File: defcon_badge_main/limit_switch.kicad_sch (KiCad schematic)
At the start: 5 parts

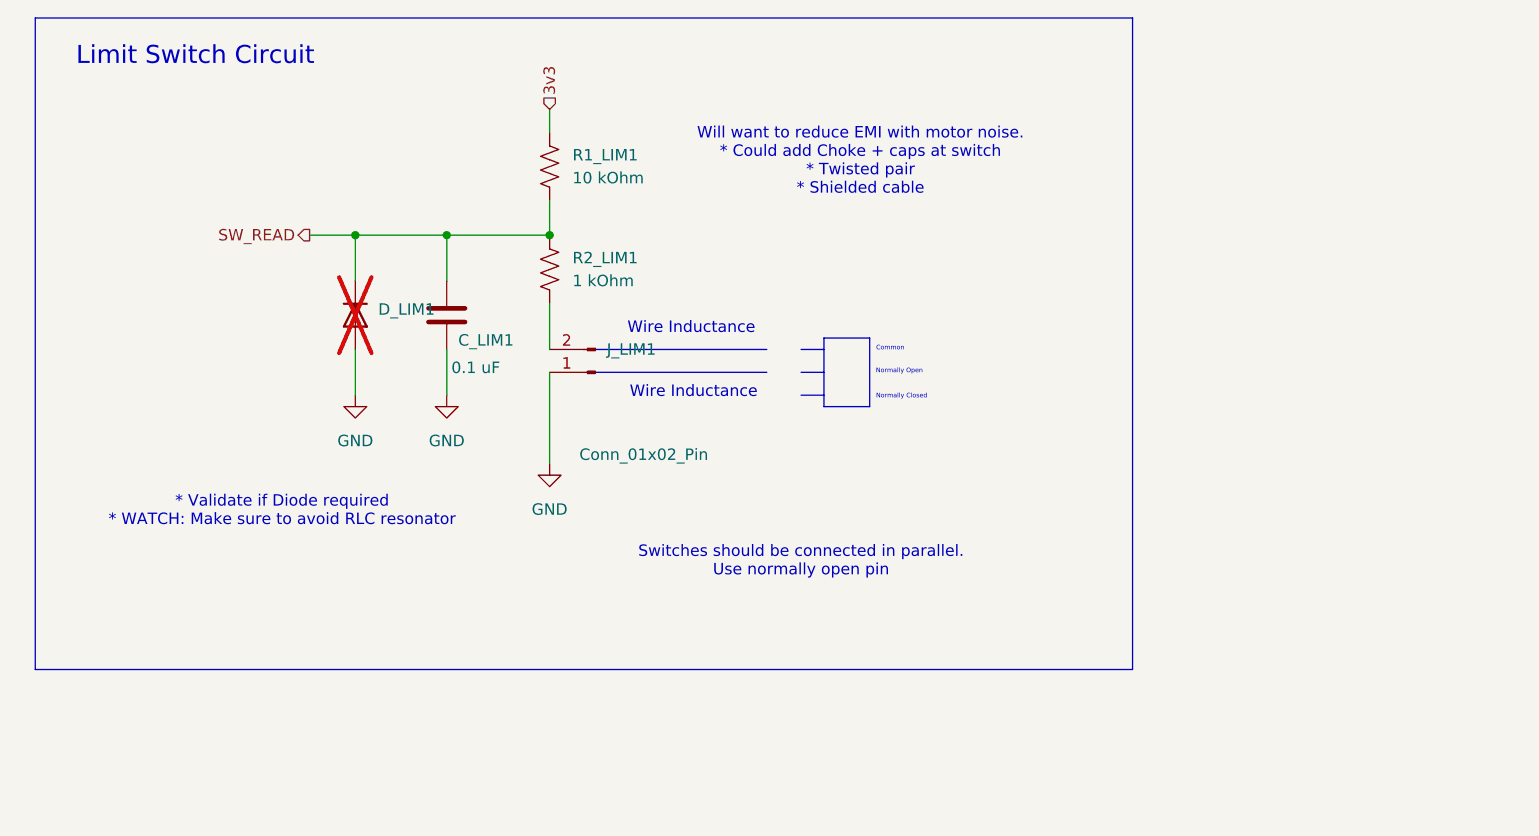
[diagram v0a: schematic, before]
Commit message: more layout
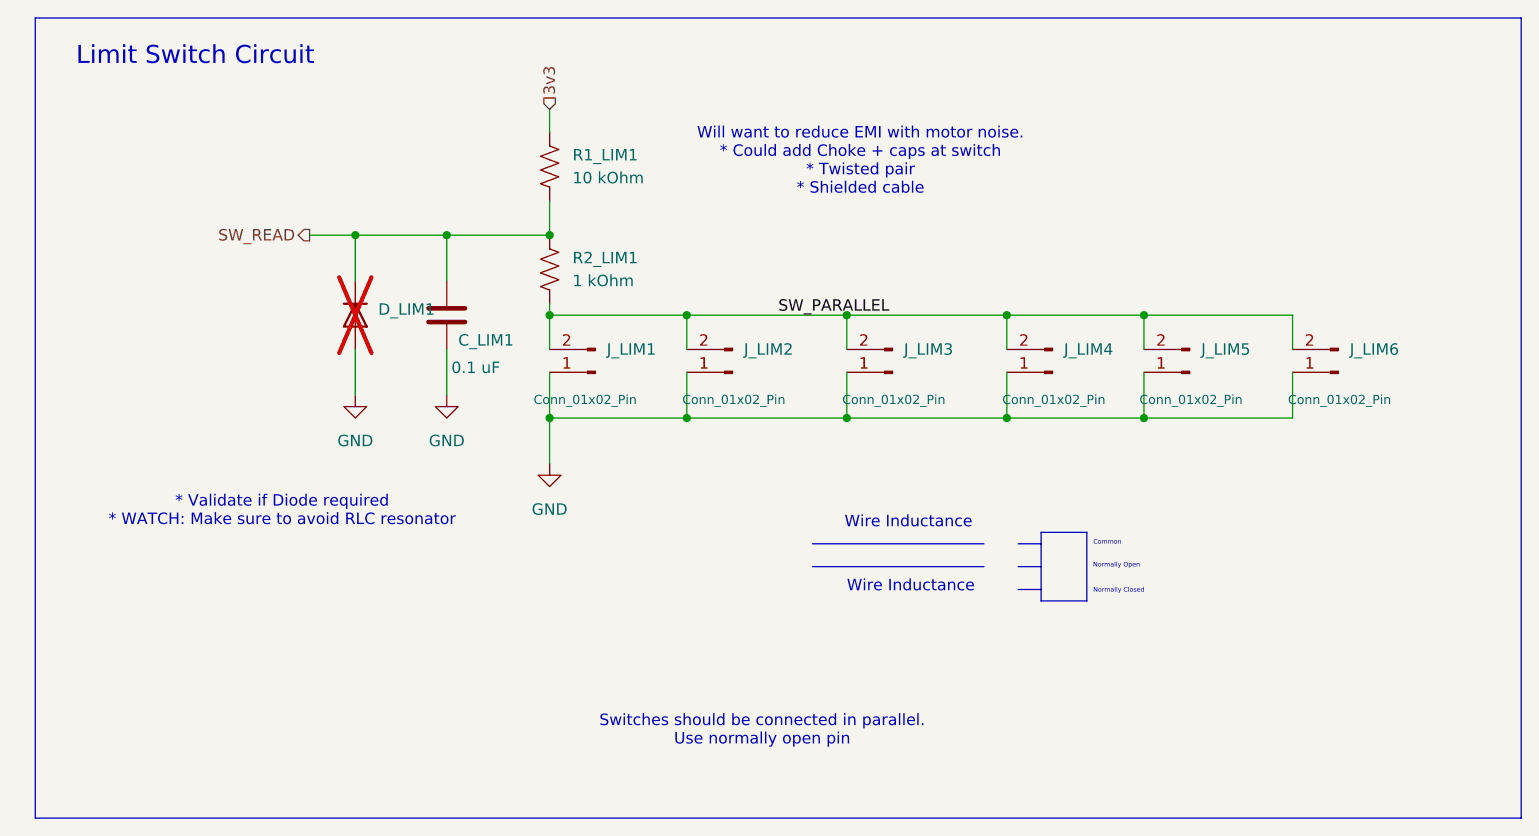
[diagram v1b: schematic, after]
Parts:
- added J_LIM2, J_LIM3, J_LIM4, J_LIM5, J_LIM6: Conn_01x02_Pin, joystick:pad_limit_switch, symbol Connector:Conn_01x02_Pin
- C_LIM1: footprint PCM_SparkFun-Coil:0805 -> joystick:R_0805_2012Metric_Pad1.20x1.40mm_HandSolder_MINE
- R1_LIM1, R2_LIM1: footprint PCM_SparkFun-Fuse:1206 -> joystick:R_1206_3216Metric_Pad1.30x1.75mm_HandSolder_MINE
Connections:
- net GND: now also J_LIM2.1 (Pin_1), J_LIM3.1 (Pin_1), J_LIM4.1 (Pin_1), J_LIM5.1 (Pin_1), J_LIM6.1 (Pin_1)
- net SW_PARALLEL: now reaches J_LIM1.2 (Pin_2), R2_LIM1.2
- net SW_PARALLEL: now also J_LIM2.2 (Pin_2), J_LIM3.2 (Pin_2), J_LIM4.2 (Pin_2), J_LIM5.2 (Pin_2), J_LIM6.2 (Pin_2)
